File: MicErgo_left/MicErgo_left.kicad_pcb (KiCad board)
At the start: 2 copper layers, 143 x 150.5 mm, 74 parts, among them J1 MJ-4PP-9, SW00 SW_Push, SW1 SW_Push, SW10 SW_Push, SW11 SW_Push, SW12 SW_Push, SW13 SW_Push, SW14 SW_Push, SW15 SW_Push, SW16 SW_Push, SW17 SW_Push, SW18 SW_Push, SW19 SW_Push, SW2 SW_Push, SW20 SW_Push, SW21 SW_Push, SW22 SW_Push, SW23 SW_Push, SW24 SW_Push, SW25 SW_Push, SW26 RotaryEncoder_Switch, SW27 SW_Push, SW28 SW_Push, SW29 SW_Push, SW3 SW_Push, SW30 SW_Push, SW31 SW_Push, SW32 SW_Push, SW4 SW_Push, SW5 SW_Push, SW6 SW_Push, SW7 SW_Push, SW8 SW_Push, SW9 SW_Push, U1 ProMicro

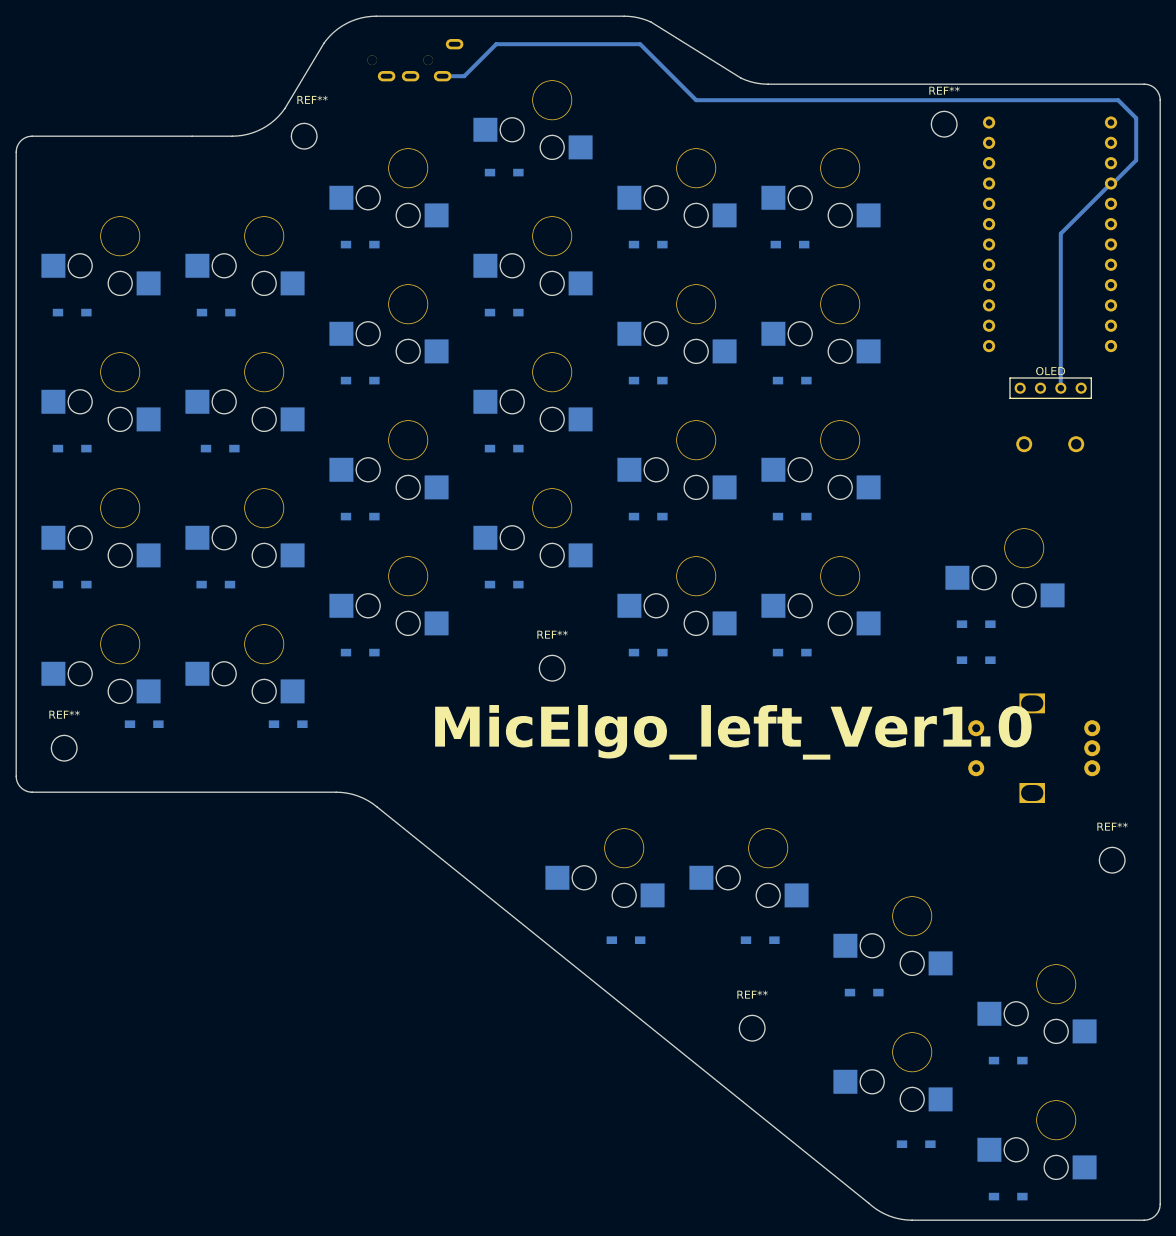
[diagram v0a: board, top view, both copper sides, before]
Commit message: Add files via upload
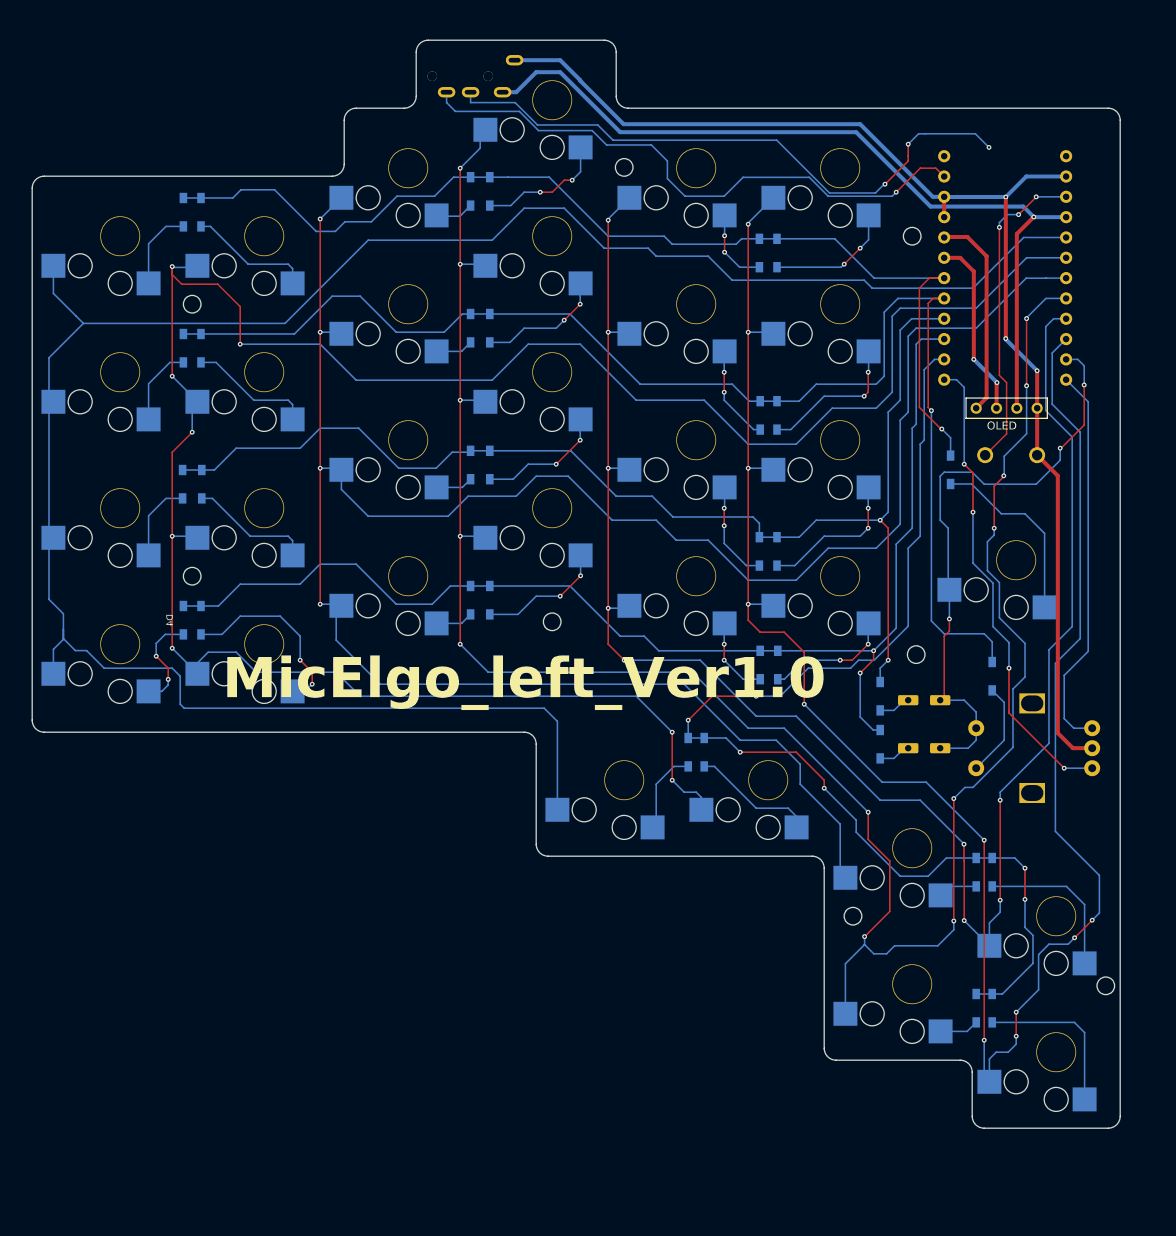
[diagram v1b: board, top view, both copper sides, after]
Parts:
- removed the D32 at (99.2, 134.0)
- removed REF** (x6): MountingHole_3.2mm_M3, MountingHole:MountingHole_3.2mm_M3
- removed the SW32 at (99.0, 122.5)
- added D26: D, my_foot:Diode_SMD_top, B.Cu at (109.0, 110.5)
- added D33: D, my_foot:Diode_SMD_top, B.Cu at (131.0, 103.5)
- added D34: D, my_foot:Diode_SMD_top, B.Cu at (131.0, 109.5)
- added Ref**: Val**, kbd_Hole:m2_Screw_Hole, F.Cu at (90.0, 94.2)
- added Ref**: Val**, kbd_Hole:m2_Screw_Hole, F.Cu at (135.5, 98.3)
- added Ref**: Val**, kbd_Hole:m2_Screw_Hole, F.Cu at (45.0, 54.5)
- added Ref**: Val**, kbd_Hole:m2_Screw_Hole, F.Cu at (159.2, 139.7)
- added Ref**: Val**, kbd_Hole:m2_Screw_Hole, F.Cu at (99.0, 37.4)
- added Ref**: Val**, kbd_Hole:m2_Screw_Hole, F.Cu at (45.0, 88.5)
- added Ref**: Val**, kbd_Hole:m2_Screw_Hole, F.Cu at (135.0, 46.0)
- added Ref**: Val**, kbd_Hole:m2_Screw_Hole, F.Cu at (127.6, 131.0)
- added SW26: SW_Push, my_foot:Choc_v2_Hotswap_1u_Narrow, B.Cu at (117.0, 114.0)
- added SW33: SW_Push, kbd_SW_PCBA:Choc_v2_予備用, B.Cu at (136.5, 104.0)
- added SW34: SW_Push, kbd_SW_PCBA:Choc_v2_予備用, B.Cu at (136.5, 110.0)
- D1, D10, D11, D12, D13, D14, D15, D16, D17, D18, D19, D2, D20, D21, D22, D23, D24, D25, D27, D28, D29, D3, D30, D31, D4, D5, D6, D7, D8, D9: footprint kbd_Parts:Diode_SMD -> my_foot:Diode_SMD_top; moved to B.Cu
- D32: renamed from D26; footprint kbd_Parts:Diode_SMD -> my_foot:Diode_SMD_top; moved to B.Cu
- J1: value MJ-4PP-9 -> TRRS_MJ-4PP-9(acid_mmVer)
- SW1, SW10, SW11, SW12, SW13, SW14, SW15, SW16, SW17, SW18, SW19, SW2, SW20, SW21, SW22, SW23, SW24, SW25, SW27, SW28, SW29, SW3, SW30, SW31, SW4, SW5, SW6, SW7, SW8, SW9: footprint kbd_SW_PCBA:Choc_v2_Hotswap_1u_Narrow -> my_foot:Choc_v2_Hotswap_1u_Narrow
- moved D31 63.4 mm to (139.8, 75.2), turned to -90 degrees
- moved SW25 57.8 mm to (99.0, 114.0)
- moved SW31 47.5 mm to (148.0, 86.5)
- moved D29 40.6 mm to (145.0, 125.5), turned to -90 degrees
- moved D25 39.4 mm to (107.0, 110.5), turned to -90 degrees
- moved SW29 25.5 mm to (153.0, 131.0)
- moved SW27 24.8 mm to (135.0, 122.5)
- moved D27 23.9 mm to (143.0, 125.5), turned to -90 degrees
- moved D30 19.5 mm to (145.0, 142.5), turned to -90 degrees
- moved D1 18.7 mm to (43.9, 43.0), turned to -90 degrees
- moved D2 18.7 mm to (43.9, 60.0), turned to -90 degrees
- moved D3 18.7 mm to (43.8, 77.0), turned to -90 degrees
- moved SW30 18.0 mm to (153.0, 148.0)
- moved D8 17.0 mm to (46.1, 94.0), turned to -90 degrees
- moved D9 15.3 mm to (79.8, 40.4), turned to -90 degrees
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- renumbered SW26 to SW32
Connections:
- D25 pad 1: row0 -> row4
- D27 pad 1: row2 -> row4
- D28 pad 1: row3 -> row4
- D29 pad 1: row0 -> row4
- D30 pad 1: row1 -> row4
- D31 pad 1: row2 -> row0
- J1 pad A: unconnected-(J1-PadA) -> GND
- J1 pad C: GND -> unconnected-(J1-PadC)
- SW25 pad 1: col6 -> col0
- SW27 pad 1: col6 -> col2
- SW28 pad 1: col6 -> col3
- SW29 pad 1: col7 -> col4
- SW30 pad 1: col7 -> col5
- SW31 pad 1: col7 -> col6
- U1 pad 10: row0 -> row3
- U1 pad 11: roA -> row4
- U1 pad 13: col7 -> roA
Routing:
- net col1: track 0.00 -> 282.5 mm, vias 0 -> 8
- net col2: track 0.00 -> 276.3 mm, vias 0 -> 4
- net col0: track 0.00 -> 272.0 mm
- net col3: track 0.00 -> 271.2 mm, vias 0 -> 13
- net col5: track 0.00 -> 247.2 mm, vias 0 -> 11
- net col4: track 0.00 -> 221.6 mm, vias 0 -> 9
- net row1: track 0.00 -> 167.8 mm, vias 0 -> 1
- net GND: track 0.00 -> 155.0 mm, vias 0 -> 3
- net row3: track 0.00 -> 151.2 mm, vias 0 -> 2
- net row2: track 0.00 -> 150.6 mm, vias 0 -> 2
- net row4: track 0.00 -> 143.7 mm, vias 0 -> 6
- net row0: track 0.00 -> 132.5 mm, vias 0 -> 1
- net unconnected-(J1-PadC): track 0.00 -> 75.9 mm, vias 0 -> 3
- net col6: track 0.00 -> 74.1 mm, vias 0 -> 3
- net DATA: track 0.00 -> 74.0 mm, vias 0 -> 1
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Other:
- board size 143 x 150.5 mm -> 136 x 136 mm
- board text added: "TRRS_C"
- board text removed: "D4"
- board text removed: "GND"
